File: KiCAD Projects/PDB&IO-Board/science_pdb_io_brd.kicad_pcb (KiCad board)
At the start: 2 copper layers, 146.1 x 94 mm, 55 parts, among them P1 PWR_IN, P11 ENCODER_1, P13 LIMIT1_IN, P14 LIMIT2_IN, P15 LIMIT3_IN, P16 ENCODER_3, P17 MOTOR1_PWM, P18 MOTOR2_PWM, P19 MOTOR3_PWM, P2 RPI_HEADER, P20 MOTOR4_PWM, P21 MOISTURE_CONN, P3 BBB_P9_HEADER, P4 BBB_P8_HEADER, P5 THERMO_SENS, P6 DIST_SENS, P7 UV_SENS, P8 ENCODER_2, U1 SN74HC14N

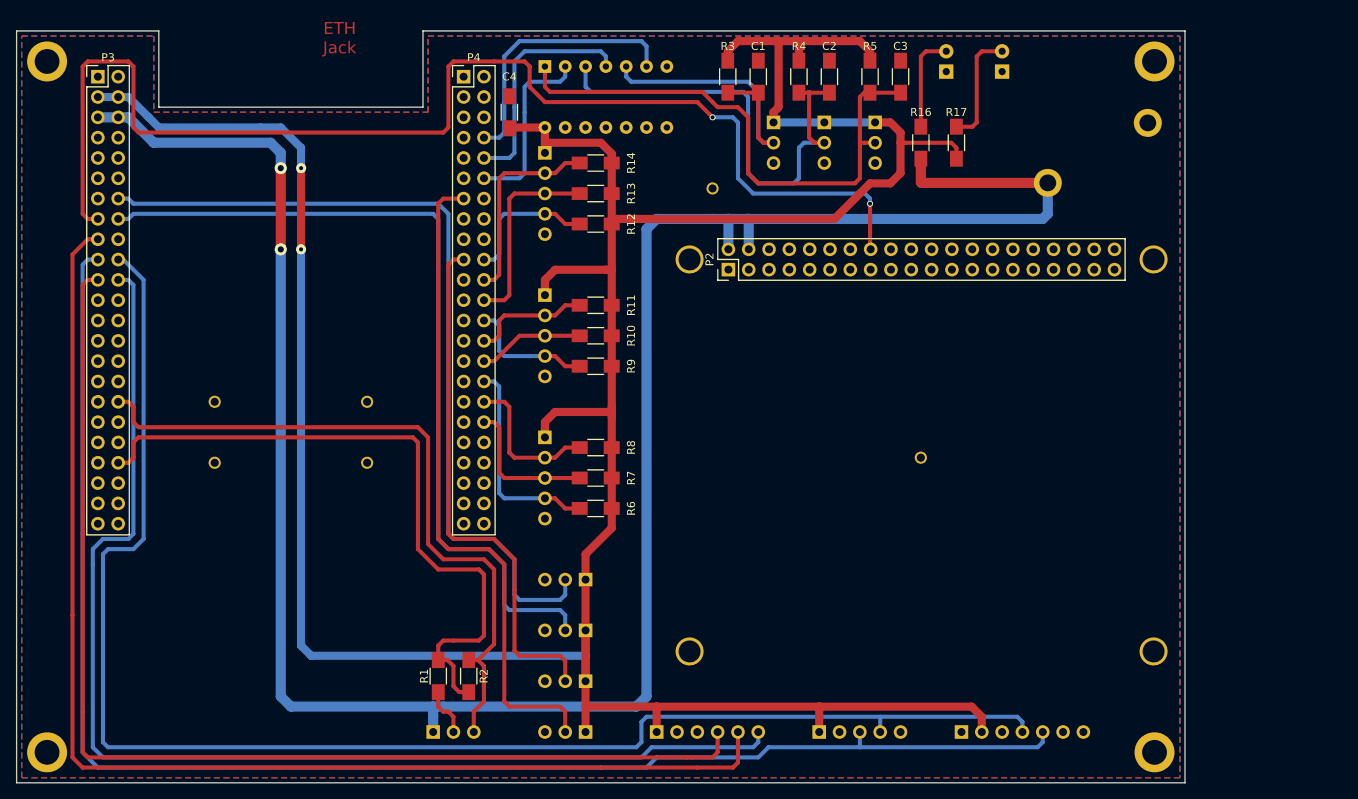
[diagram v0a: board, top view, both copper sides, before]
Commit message: Made CHanges to Raspberry Pi
These definitely are not wrong at all.
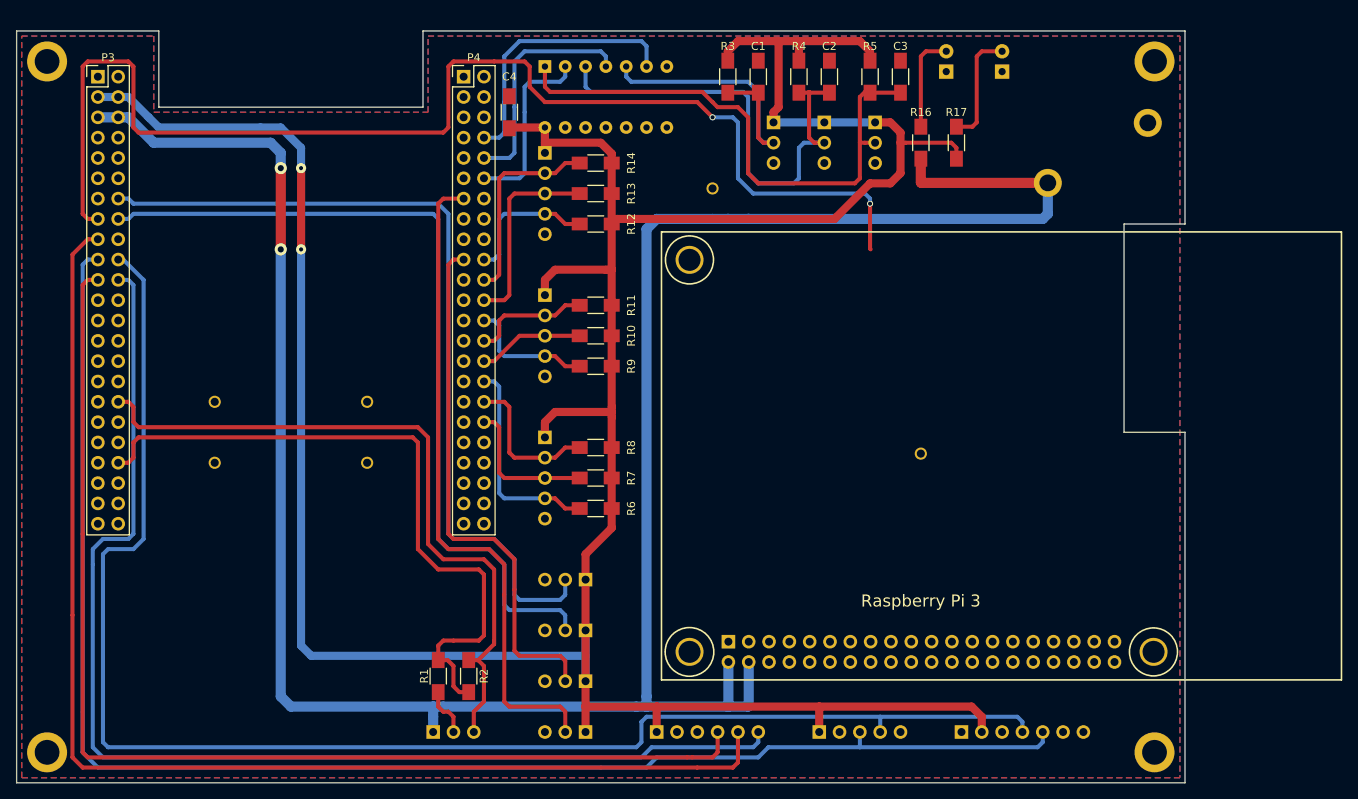
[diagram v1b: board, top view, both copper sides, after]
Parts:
- P2, REF** (x5): moved to B.Cu
- moved REF** 49.1 mm to (178.9, 99.2)
- moved REF** 49.1 mm to (121.0, 99.2)
- moved REF** 48.9 mm to (178.9, 50.2)
- moved REF** 48.9 mm to (121.0, 50.2)
- moved P2 46.5 mm to (125.8, 97.9), turned to 270 degrees
- moved REF** 0.51 mm to (149.9, 74.4)
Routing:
- net +5V: track 282.5 -> 299.6 mm
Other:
- outline, holes or cut-outs redrawn
- board text removed: "ETH Jack"

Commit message: Revert "Made CHanges to Raspberry Pi"
This reverts commit 9b6c6e1ff9c729eb0e6bf7611c964737bcdfa00b.
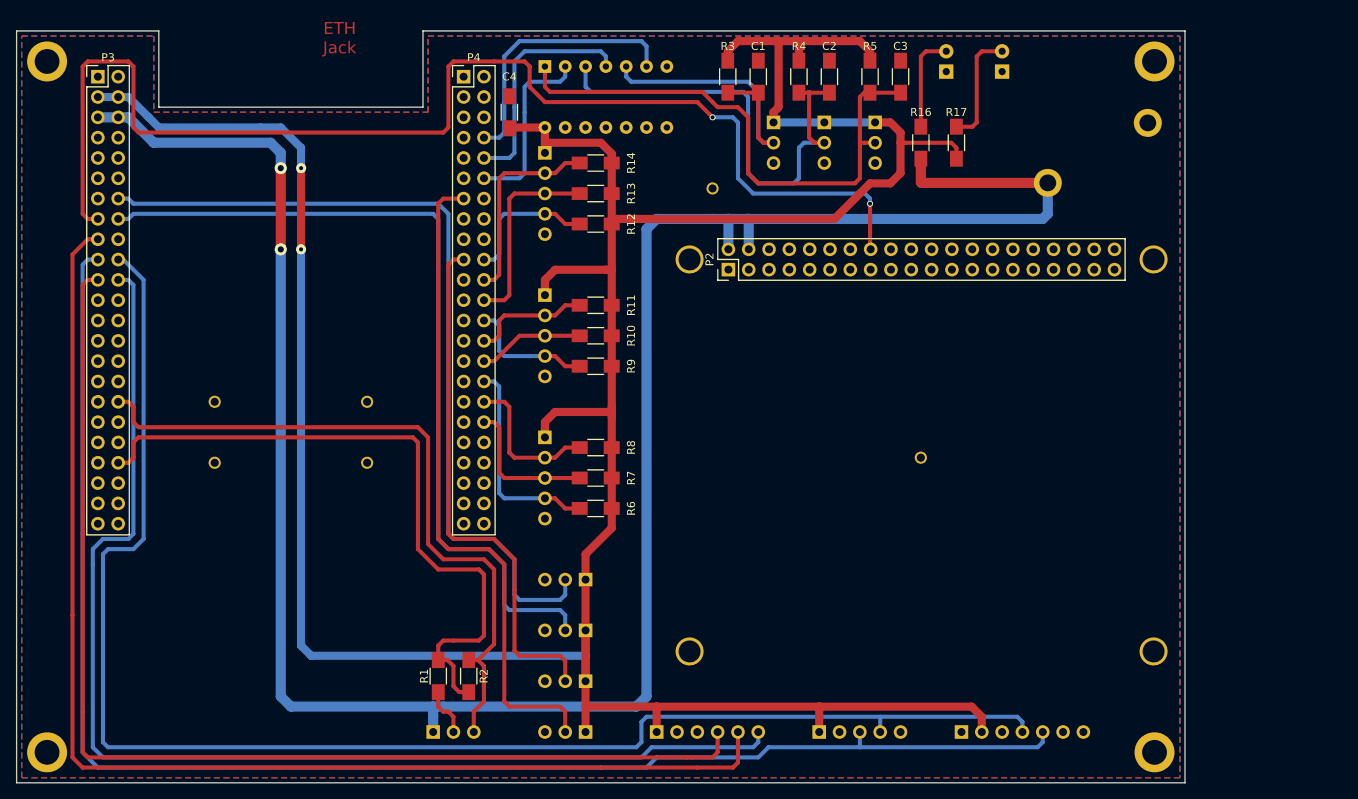
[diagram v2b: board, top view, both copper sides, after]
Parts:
- P2, REF** (x5): moved to F.Cu
- moved REF** 49.1 mm to (178.9, 50.1)
- moved REF** 49.1 mm to (121.0, 50.1)
- moved REF** 48.9 mm to (178.9, 99.2)
- moved REF** 48.9 mm to (121.0, 99.2)
- moved P2 46.5 mm to (125.8, 51.4), turned to 90 degrees
- moved REF** 0.51 mm to (149.9, 74.9)
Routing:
- net +5V: track 299.6 -> 282.5 mm
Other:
- outline, holes or cut-outs redrawn
- board text added: "ETH Jack"
